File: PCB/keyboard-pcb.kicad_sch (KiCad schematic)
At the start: 181 parts, among them J1 Conn_01x05_Pin, U1 Raspberry_Pi_Pico

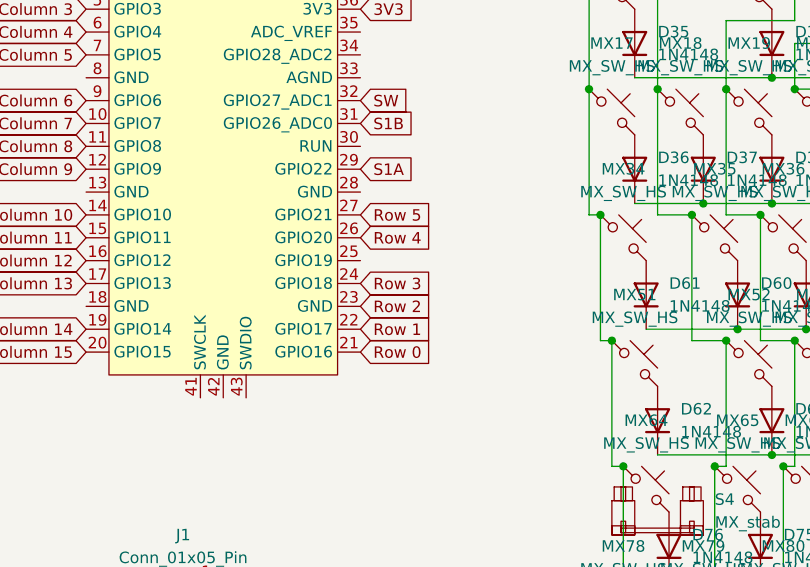
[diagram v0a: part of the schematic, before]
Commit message: Modified JOURNAL.md
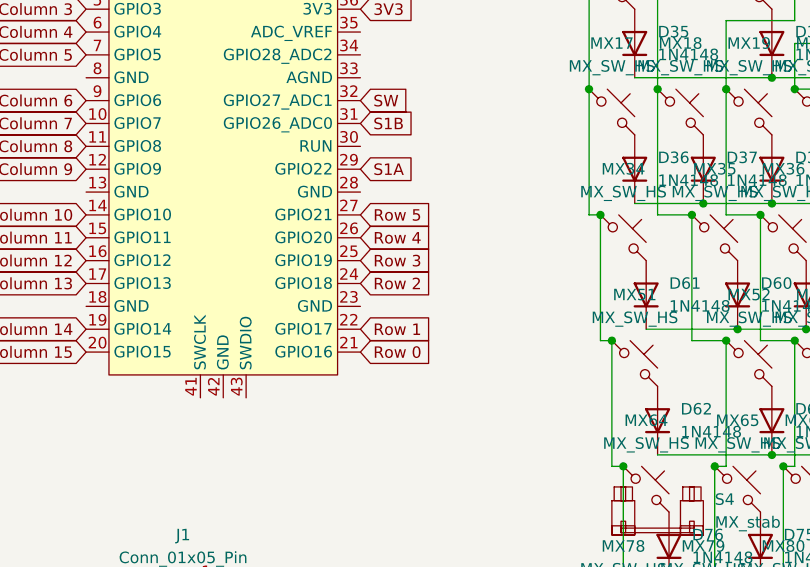
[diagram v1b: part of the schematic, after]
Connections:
- net Row 2: now also U1.24 (GPIO18); no longer U1.23 (GND)
- net Row 3: now also U1.25 (GPIO19); no longer U1.24 (GPIO18)
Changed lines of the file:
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@@
 	(global_label "Row 3"
 		(shape input)
-		(at 60.96 64.77 0)
+		(at 60.96 62.23 0)
 		(fields_autoplaced yes)
 		(effects
@@
 		)
 		(property "Intersheetrefs" "${INTERSHEET_REFS}"
-			(at 69.8718 64.77 0)
+			(at 69.8718 62.23 0)
 			(effects
 				(font
@@
 	(global_label "Row 2"
 		(shape input)
-		(at 60.96 67.31 0)
+		(at 60.96 64.77 0)
 		(fields_autoplaced yes)
 		(effects
@@
 		)
 		(property "Intersheetrefs" "${INTERSHEET_REFS}"
-			(at 69.8718 67.31 0)
+			(at 69.8718 64.77 0)
 			(effects
 				(font
